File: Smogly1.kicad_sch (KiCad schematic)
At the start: 10 parts, among them J1 VCC IN, J10 NodeMCU A0-VIN, J11 NodeMCU D0-3.3V, J2 PMSx003, J3 BME280, J4 microUSB, J5 5/3.3/GND, J6 DeepSleep, J8 D5/6/7/8, J9 PMS7003_Conn

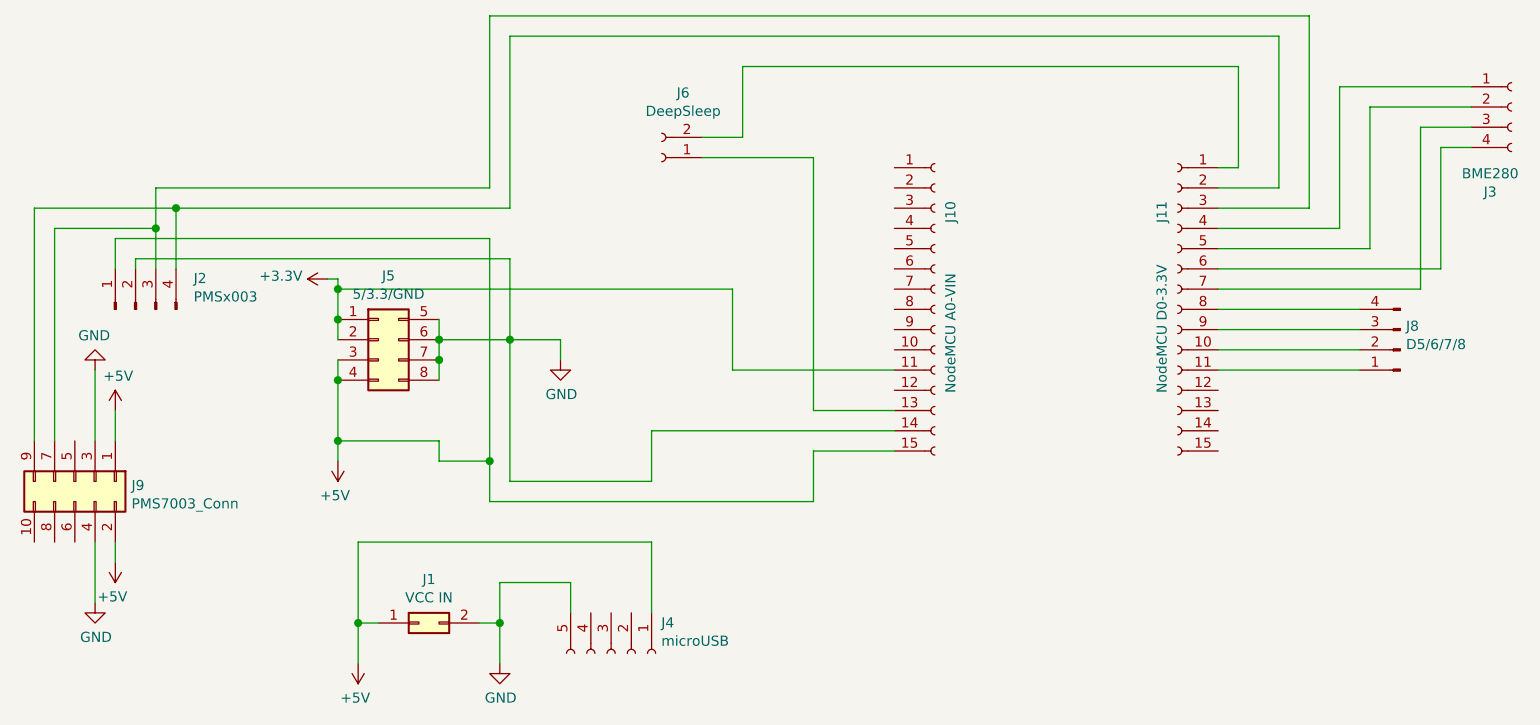
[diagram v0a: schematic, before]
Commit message: KiCad 6.0
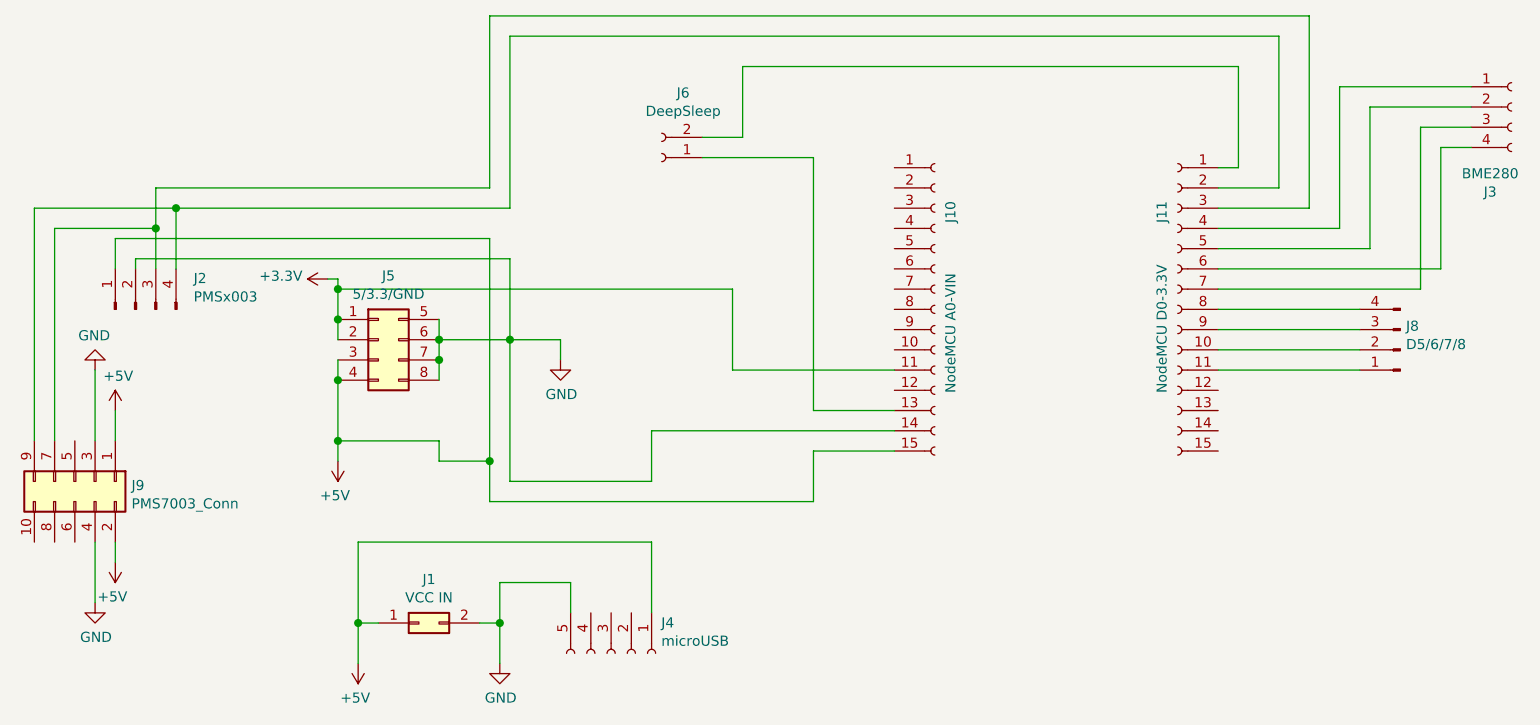
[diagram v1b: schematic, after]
